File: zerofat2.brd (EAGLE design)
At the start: 50 x 50 mm, 54 parts, among them IC1 MCP1703T-3302E/CB

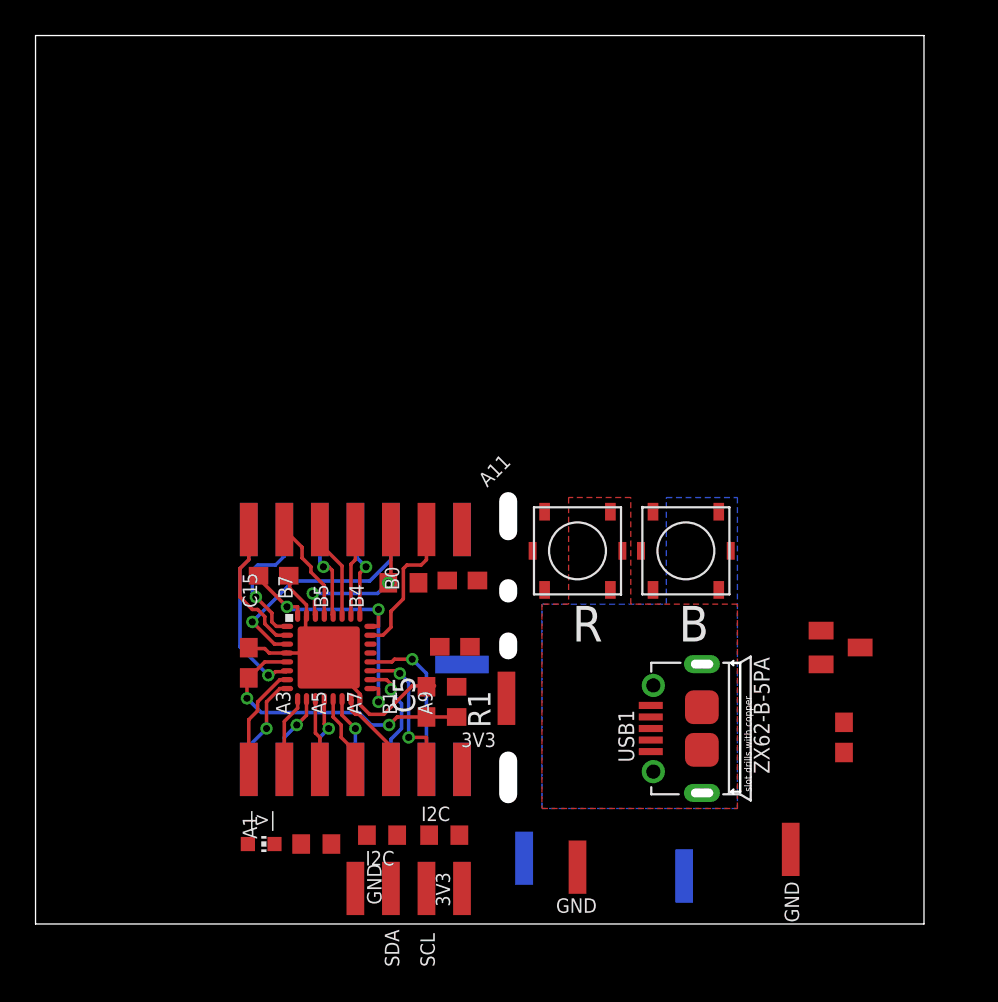
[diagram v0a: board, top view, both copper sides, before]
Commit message: ZeroFat32 v2 (STM32L082)
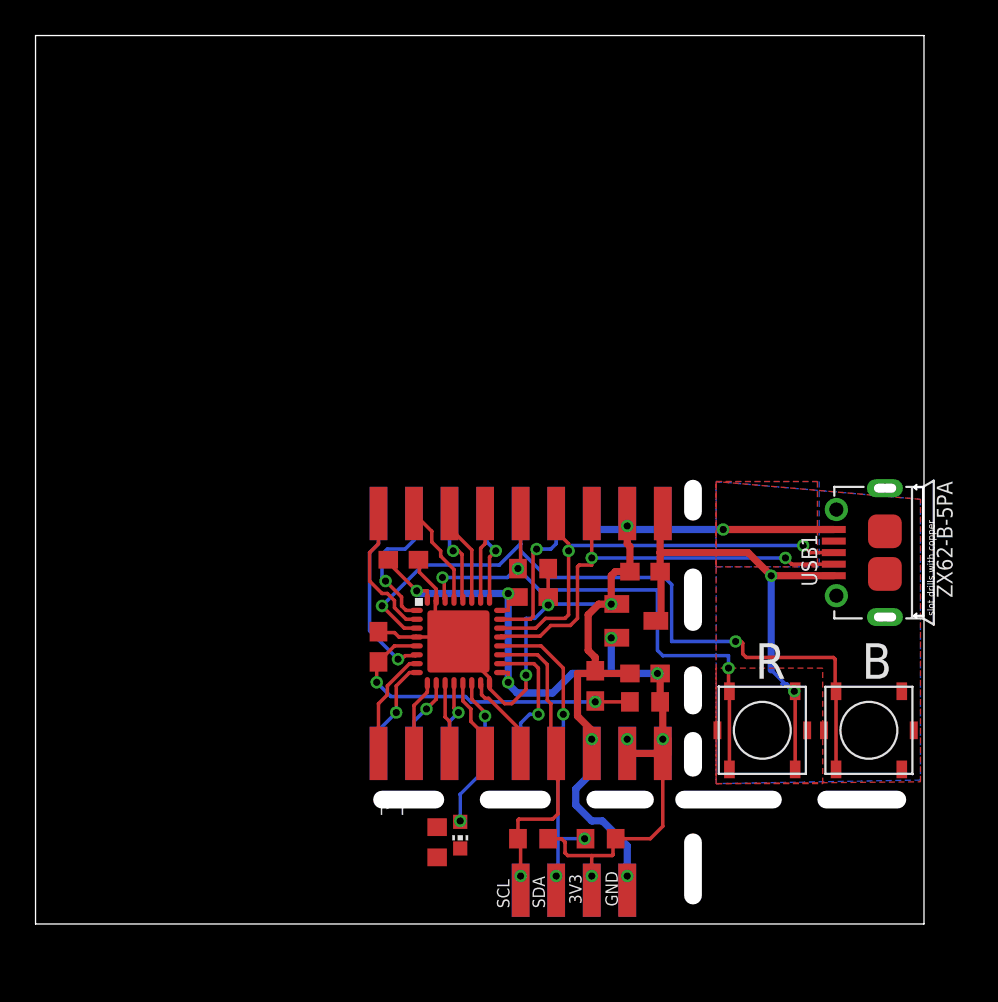
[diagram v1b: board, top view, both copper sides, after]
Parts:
- added PAD15, PAD21, PAD7: 3V3, zerofat:PAD_MINIMAL
- added PAD19: SDA, zerofat:PAD_MINIMAL
- added PAD20: SCL, zerofat:PAD_MINIMAL
- added PAD22, PAD5: GND, zerofat:PAD_MINIMAL
- PAD35: value B0 -> BL
- PAD43, PAD48: value 3V3 -> GND
- moved PAD50 22.0 mm to (31.3, 23.1), flipped to the bottom
- moved PAD39 20.6 mm to (33.3, 23.1)
- moved PAD49 20.1 mm to (33.3, 23.1)
- moved R 19.3 mm to (46.9, 10.9)
- moved C3 19.2 mm to (28.0, 18.4), turned to 0 degrees
- moved PAD51 15.3 mm to (33.3, 1.90)
- moved USB1 14.3 mm to (47.8, 20.9)
- moved PAD45 14.1 mm to (35.3, 23.1), flipped to the top, turned to 0 degrees
- moved R3 12.3 mm to (31.8, 4.80)
- moved IC1 11.6 mm to (33.8, 17.1)
- moved LED1 11.2 mm to (23.9, 5.00), turned to 180 degrees
- moved B 11.0 mm to (40.9, 10.9)
- moved C6 10.8 mm to (34.3, 14.1)
- moved R1 10.6 mm to (34.3, 12.5), turned to 180 degrees
- moved C1 10.3 mm to (34.3, 19.8)
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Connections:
- net N$43 renamed BOOT0
- net +3V3: now also PAD15.1, PAD21.1, PAD7.1; no longer PAD43.1, PAD48.1
- net GND: now also PAD22.1, PAD43.1, PAD48.1, PAD5.1
- net N$21: now also PAD20.1
- net N$23: now also PAD19.1
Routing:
- net GND: track 18.5 -> 75.0 mm, vias 0 -> 7
- net +3V3: track 16.8 -> 54.4 mm, vias 3 -> 8
- net +5V: track 0.00 -> 29.7 mm, vias 0 -> 2
- net N$45: track 13.4 -> 42.5 mm, vias 1 -> 2
- net N$4: track 0.00 -> 25.4 mm, vias 0 -> 2
- net N$1: track 0.00 -> 25.2 mm, vias 0 -> 2
- net BOOT0: track 8.87 -> 31.3 mm, vias 2 -> 3
- net N$21: track 8.32 -> 18.9 mm, vias 2 -> 1
- net N$23: track 8.94 -> 19.2 mm, vias 1 -> 3
- net N$2: track 4.26 -> 8.69 mm, vias 1 -> 2
- net VCCINT: track 16.3 -> 18.5 mm
- net N$19: track 6.55 -> 7.76 mm
- net N$3: track 8.20 -> 8.79 mm, vias 0 -> 1
- added copper zone on layer 1, net N$24
- added copper zone on layer 1, net N$25
- added copper zone on layer 16, net N$26
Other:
- outline, holes or cut-outs redrawn
- board text added: "3V3"
- board text added: "5V/GND"
- board text added: "A1/A2"
- board text added: "A11/GND"
- board text added: "A12/A13"
- board text added: "A3/A4"
- board text added: "A5/A6"
- board text added: "A7/B0"
- board text added: "A9/A10"
- board text added: "B1/A8"
- board text added: "B4/A14"
- board text added: "B5/B6"
- board text added: "B7/C14"
- board text added: "BOOT/!R"
- board text added: "C15/A0"
- board text added: "GND"
- board text added: "http://elmot.xyz/"
- board text removed: "http://elmot.github.io/"
